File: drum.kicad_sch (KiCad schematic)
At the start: 39 parts, among them J101 Cortex_Debug, J102 DX07S016JA3, SW101 SKSG, SW102 SKSG, U101 ATSAMD51J, U102 TPS78433QWDRBRQ1, Y101 32k768

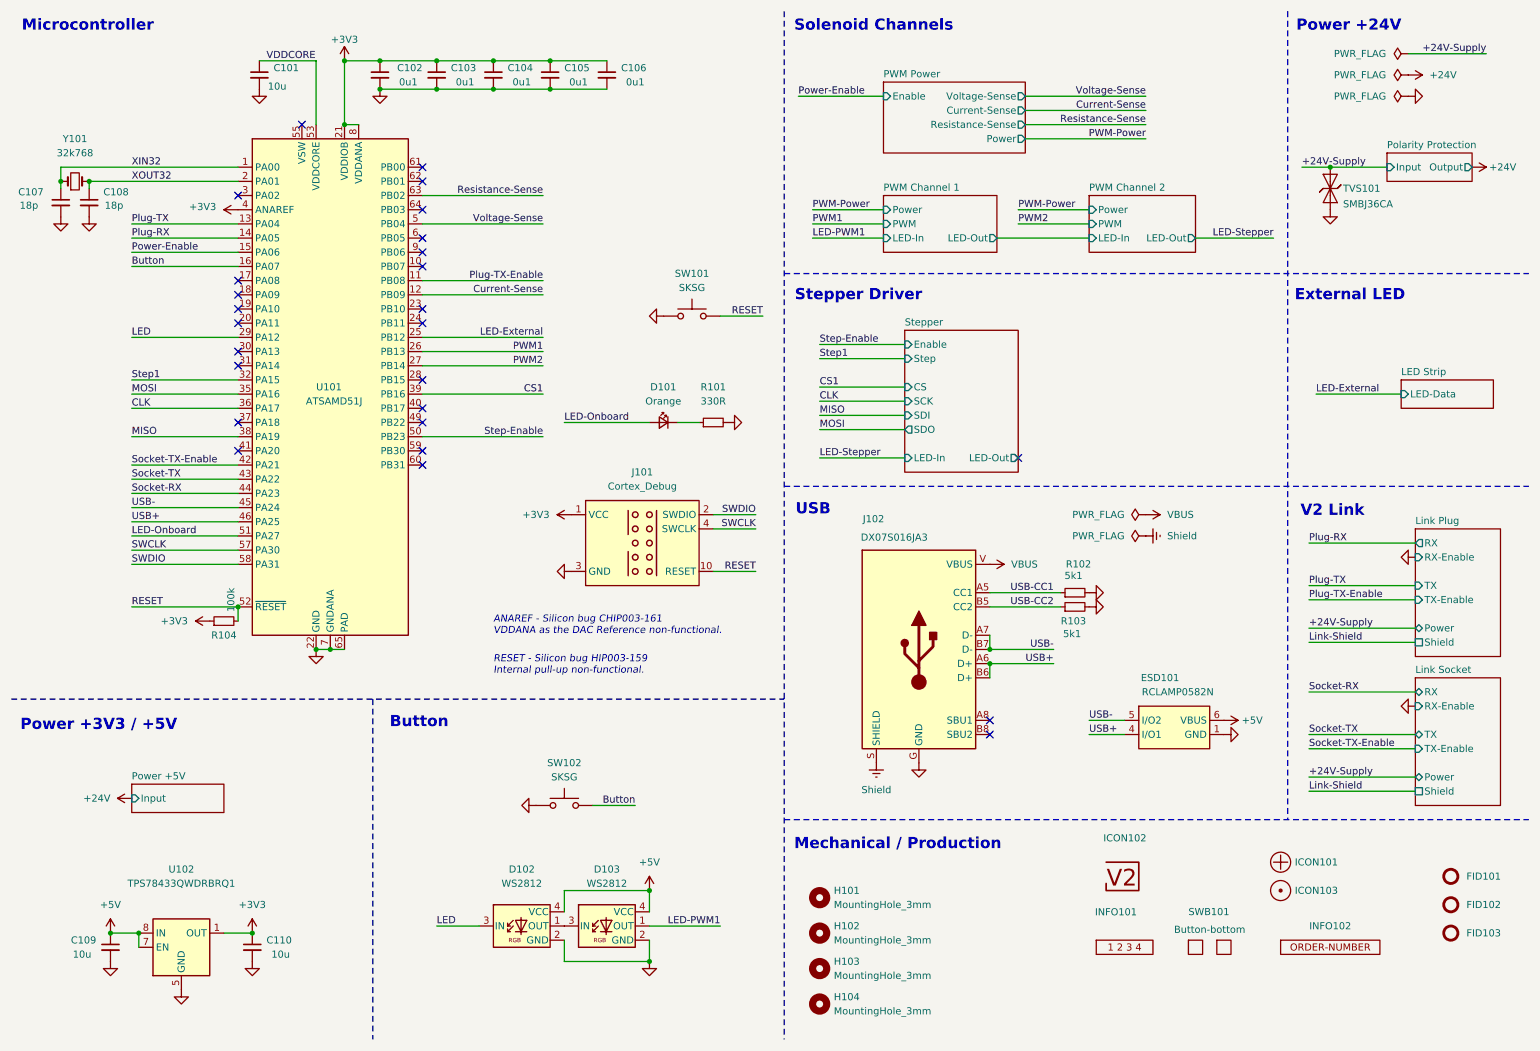
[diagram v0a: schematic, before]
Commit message: Update library
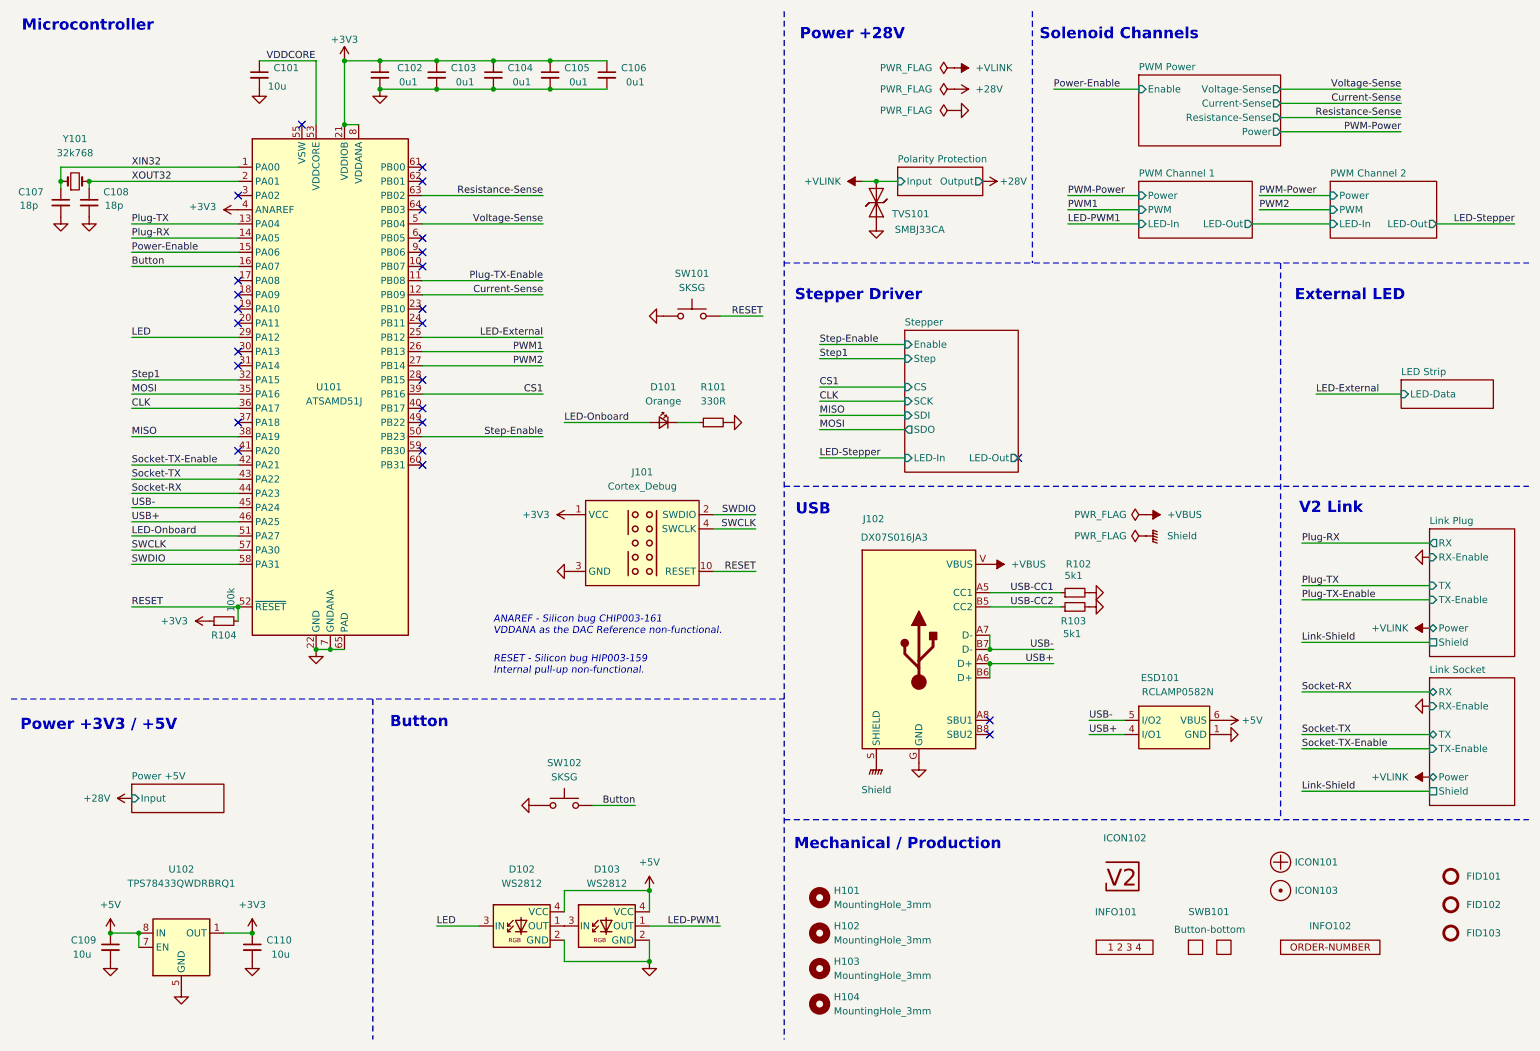
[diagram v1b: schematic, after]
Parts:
- C101: Rating (none) -> 10V
- C102, C103, C104, C105, C106: Rating (none) -> 50V
- D101: Mouser 755-SML-D12M8WT86C -> 755-SML-D12D1WT86; Product SML-D12M8WT86C -> SML-D12D1WT86
- TVS101: value SMBJ36CA -> SMBJ33CA; symbol V2_Diode:SMBJ36CA -> V2_Diode:SMBJ33CA; Mouser 652-SMBJ36CA-Q -> 652-SMBJ33CA-Q; Product SMBJ36CA-Q -> SMBJ33CA-Q; Rating 36V -> 33V
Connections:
- net +24V-Supply renamed +VLINK
- net VBUS renamed +VBUS
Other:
- note added: "Power +28V"
- note removed: "Power +24V"
- moved on the sheet: TVS101
